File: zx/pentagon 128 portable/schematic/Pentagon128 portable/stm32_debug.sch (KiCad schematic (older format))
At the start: 4 parts, among them J3 Conn_ARM_JTAG_SWD_20

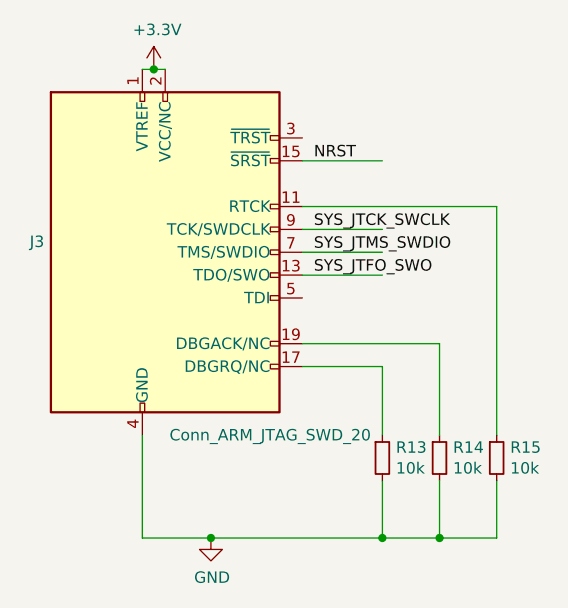
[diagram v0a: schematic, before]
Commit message: updated BOM
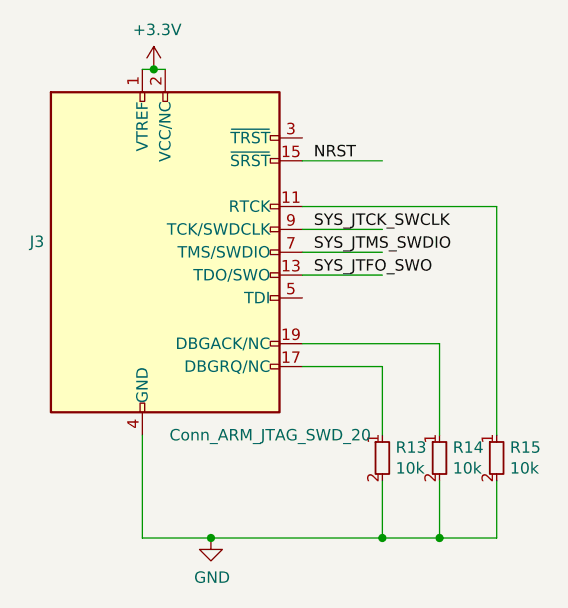
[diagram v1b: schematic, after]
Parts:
- removed R13, R14, R15: 10k, Resistor_SMD:R_0402_1005Metric, symbol Device:R_Small
- added R13, R14, R15: 10k, RESC1005X37N, symbol SamacSys_Parts:10k
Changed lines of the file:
@@
 Wire Wire Line
 	3600 5000 3900 5000
-$Comp
-L Device:R_Small R15
-U 1 1 5F9AFF8C
-P 5150 4650
-F 0 "R15" H 5209 4696 50  0000 L CNN
-F 1 "10k" H 5209 4605 50  0000 L CNN
-F 2 "Resistor_SMD:R_0402_1005Metric" H 5150 4650 50  0001 C CNN
-F 3 "~" H 5150 4650 50  0001 C CNN
-	1    5150 4650
-	1    0    0    -1
-$EndComp
-$Comp
-L Device:R_Small R14
-U 1 1 5F9AFF92
-P 4900 4650
-F 0 "R14" H 4959 4696 50  0000 L CNN
-F 1 "10k" H 4959 4605 50  0000 L CNN
-F 2 "Resistor_SMD:R_0402_1005Metric" H 4900 4650 50  0001 C CNN
-F 3 "~" H 4900 4650 50  0001 C CNN
-	1    4900 4650
-	1    0    0    -1
-$EndComp
-$Comp
-L Device:R_Small R13
-U 1 1 5F9AFF98
-P 4650 4650
-F 0 "R13" H 4709 4696 50  0000 L CNN
-F 1 "10k" H 4709 4605 50  0000 L CNN
-F 2 "Resistor_SMD:R_0402_1005Metric" H 4650 4650 50  0001 C CNN
-F 3 "~" H 4650 4650 50  0001 C CNN
-	1    4650 4650
-	1    0    0    -1
-$EndComp
 Wire Wire Line
 	5150 4550 5150 3550
@@
 	5150 5000 4900 5000
 Connection ~ 4900 5000
+$Comp
+L SamacSys_Parts:10k R13
+U 1 1 5F90C9DC
+P 4650 4650
+F 0 "R13" H 4708 4696 50  0000 L CNN
+F 1 "10k" H 4708 4605 50  0000 L CNN
+F 2 "RESC1005X37N" H 4700 4500 50  0001 L CNN
+F 3 "https://componentsearchengine.com/Datasheets/1/MCS0402MC1002FE000.pdf" H 4700 4400 50  0001 L CNN
+F 4 "Thin Film Resistors - SMD .1W 10Kohms 1% 0402 50ppm Auto" H 4700 4300 50  0001 L CNN "Description"
+F 5 "0.37" H 4700 4200 50  0001 L CNN "Height"
+F 6 "594-MCS0402MC1002FE0" H 4700 4100 50  0001 L CNN "Mouser Part Number"
+F 7 "https://www.mouser.com/Search/Refine.aspx?Keyword=594-MCS0402MC1002FE0" H 4700 4000 50  0001 L CNN "Mouser Price/Stock"
+F 8 "Vishay" H 4700 3900 50  0001 L CNN "Manufacturer_Name"
+F 9 "MCS0402MC1002FE000" H 4700 3800 50  0001 L CNN "Manufacturer_Part_Number"
+	1    4650 4650
+	1    0    0    -1
+$EndComp
+$Comp
+L SamacSys_Parts:10k R14
+U 1 1 5F90D320
+P 4900 4650
+F 0 "R14" H 4958 4696 50  0000 L CNN
+F 1 "10k" H 4958 4605 50  0000 L CNN
+F 2 "RESC1005X37N" H 4950 4500 50  0001 L CNN
+F 3 "https://componentsearchengine.com/Datasheets/1/MCS0402MC1002FE000.pdf" H 4950 4400 50  0001 L CNN
+F 4 "Thin Film Resistors - SMD .1W 10Kohms 1% 0402 50ppm Auto" H 4950 4300 50  0001 L CNN "Description"
+F 5 "0.37" H 4950 4200 50  0001 L CNN "Height"
+F 6 "594-MCS0402MC1002FE0" H 4950 4100 50  0001 L CNN "Mouser Part Number"
+F 7 "https://www.mouser.com/Search/Refine.aspx?Keyword=594-MCS0402MC1002FE0" H 4950 4000 50  0001 L CNN "Mouser Price/Stock"
+F 8 "Vishay" H 4950 3900 50  0001 L CNN "Manufacturer_Name"
+F 9 "MCS0402MC1002FE000" H 4950 3800 50  0001 L CNN "Manufacturer_Part_Number"
+	1    4900 4650
+	1    0    0    -1
+$EndComp
+$Comp
+L SamacSys_Parts:10k R15
+U 1 1 5F90D64E
+P 5150 4650
+F 0 "R15" H 5208 4696 50  0000 L CNN
+F 1 "10k" H 5208 4605 50  0000 L CNN
+F 2 "RESC1005X37N" H 5200 4500 50  0001 L CNN
+F 3 "https://componentsearchengine.com/Datasheets/1/MCS0402MC1002FE000.pdf" H 5200 4400 50  0001 L CNN
+F 4 "Thin Film Resistors - SMD .1W 10Kohms 1% 0402 50ppm Auto" H 5200 4300 50  0001 L CNN "Description"
+F 5 "0.37" H 5200 4200 50  0001 L CNN "Height"
+F 6 "594-MCS0402MC1002FE0" H 5200 4100 50  0001 L CNN "Mouser Part Number"
+F 7 "https://www.mouser.com/Search/Refine.aspx?Keyword=594-MCS0402MC1002FE0" H 5200 4000 50  0001 L CNN "Mouser Price/Stock"
+F 8 "Vishay" H 5200 3900 50  0001 L CNN "Manufacturer_Name"
+F 9 "MCS0402MC1002FE000" H 5200 3800 50  0001 L CNN "Manufacturer_Part_Number"
+	1    5150 4650
+	1    0    0    -1
+$EndComp
 $EndSCHEMATC
